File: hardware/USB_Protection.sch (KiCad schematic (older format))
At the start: 10 parts, among them Q1 DMN6140L, U12 TCPP01-M12

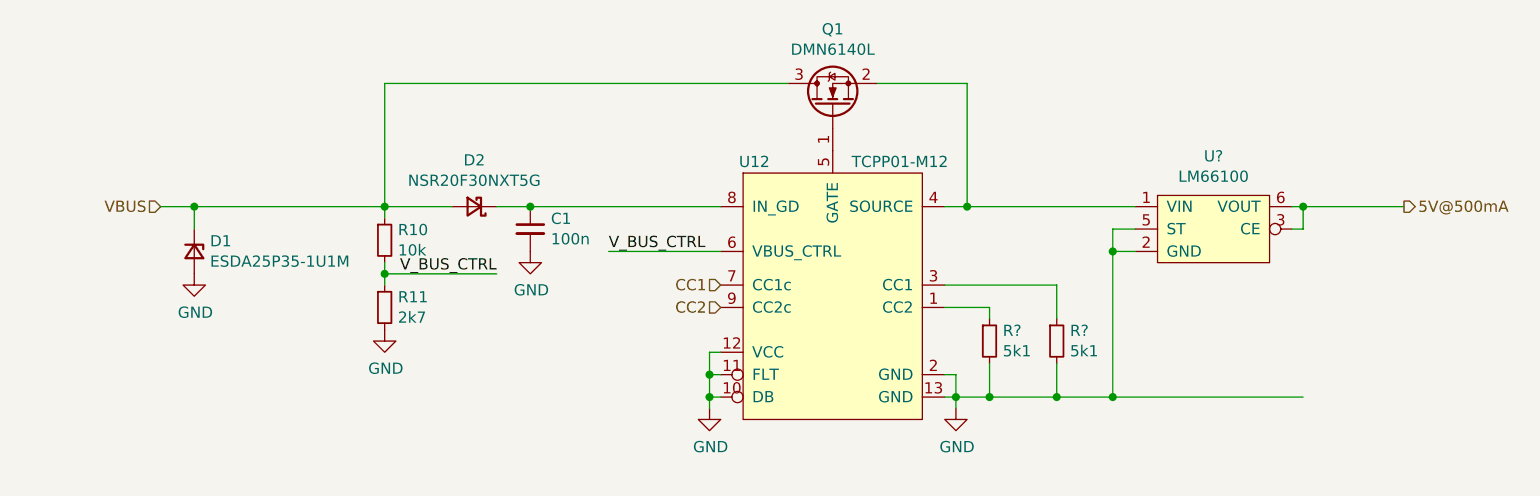
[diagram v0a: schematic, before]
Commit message: hardware development
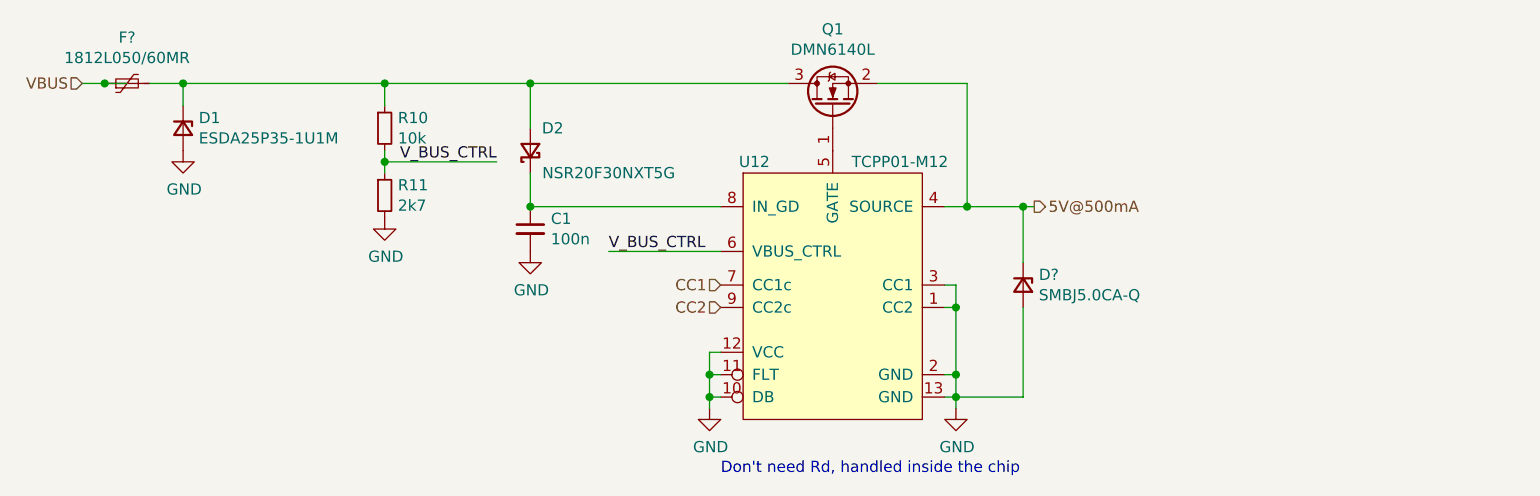
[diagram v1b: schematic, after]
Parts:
- removed R? (x2): 5k1, Resistor_SMD:R_0603_1608Metric_Pad1.05x0.95mm_HandSolder, symbol Device:R_Small
- removed U?: LM66100, lm66100:LM66100DCKT, symbol watch:LM66100-Variant2
- added D?: SMBJ5.0CA-Q, Diode_SMD:D_0603_1608Metric_Pad1.05x0.95mm_HandSolder, symbol Device:D_Zener_Small
- added F?: 1812L050/60MR, symbol Device:Polyfuse_Small
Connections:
- wire segments 45 -> 37
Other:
- note added: "Don't need Rd, handled inside the chip"
- moved on the sheet: D1, D2, R10, R11
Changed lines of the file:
@@
 $Descr A4 11693 8268
 encoding utf-8
-Sheet 2 3
+Sheet 3 4
 Title ""
 Date ""
@@
 AR Path="/6072C21E" Ref="U?"  Part="1"
 AR Path="/6071FFAF/6072C21E" Ref="U12"  Part="1"
+AR Path="/60604F0C/6060934C/6072C21E" Ref="U?"  Part="1"
 F 0 "U12" H 4650 3750 50  0000 C CNN
 F 1 "TCPP01-M12" H 5300 3750 50  0000 C CNN
@@
 L Device:D_Zener_Small D?
 U 1 1 60731C37
-P 2150 2950
+P 2100 2400
 AR Path="/60731C37" Ref="D?"  Part="1"
 AR Path="/6071FFAF/60731C37" Ref="D1"  Part="1"
-F 0 "D1" V 2104 3020 50  0000 L CNN
-F 1 "ESDA25P35-1U1M" V 2195 3020 50  0000 L CNN
-F 2 "Diode_SMD:D_0603_1608Metric_Pad1.05x0.95mm_HandSolder" V 2150 2950 50  0001 C CNN
-F 3 "~" V 2150 2950 50  0001 C CNN
-	1    2150 2950
+AR Path="/60604F0C/6060934C/60731C37" Ref="D?"  Part="1"
+F 0 "D1" V 2054 2470 50  0000 L CNN
+F 1 "ESDA25P35-1U1M" V 2145 2470 50  0000 L CNN
+F 2 "Diode_SMD:D_0603_1608Metric_Pad1.05x0.95mm_HandSolder" V 2100 2400 50  0001 C CNN
+F 3 "~" V 2100 2400 50  0001 C CNN
+	1    2100 2400
 	0    1    1    0
 $EndComp
-Text HLabel 2000 2750 0    50   Input ~ 0
+Text HLabel 1650 2200 0    50   Input ~ 0
 VBUS
 Text HLabel 4500 3100 0    50   Input ~ 0
@@
 U 1 1 605BE08D
 P 5550 3650
+AR Path="/6071FFAF/605BE08D" Ref="#PWR0130"  Part="1"
+AR Path="/60604F0C/6060934C/605BE08D" Ref="#PWR?"  Part="1"
 F 0 "#PWR0130" H 5550 3400 50  0001 C CNN
 F 1 "GND" H 5555 3477 50  0000 C CNN
@@
 U 1 1 605BEA49
 P 4450 3650
+AR Path="/6071FFAF/605BEA49" Ref="#PWR0131"  Part="1"
+AR Path="/60604F0C/6060934C/605BEA49" Ref="#PWR?"  Part="1"
 F 0 "#PWR0131" H 4450 3400 50  0001 C CNN
 F 1 "GND" H 4455 3477 50  0000 C CNN
@@
 	4450 3600 4450 3500
 Wire Wire Line
-	2150 2850 2150 2750
-Wire Wire Line
-	2150 2750 2000 2750
+	2100 2300 2100 2200
 $Comp
 L Device:R_Small R10
 U 1 1 605BF926
-P 3000 2900
-F 0 "R10" H 3059 2946 50  0000 L CNN
-F 1 "10k" H 3059 2855 50  0000 L CNN
-F 2 "Resistor_SMD:R_0603_1608Metric_Pad1.05x0.95mm_HandSolder" H 3000 2900 50  0001 C CNN
-F 3 "~" H 3000 2900 50  0001 C CNN
-	1    3000 2900
+P 3000 2400
+AR Path="/6071FFAF/605BF926" Ref="R10"  Part="1"
+AR Path="/60604F0C/6060934C/605BF926" Ref="R?"  Part="1"
+F 0 "R10" H 3059 2446 50  0000 L CNN
+F 1 "10k" H 3059 2355 50  0000 L CNN
+F 2 "Resistor_SMD:R_0603_1608Metric_Pad1.05x0.95mm_HandSolder" H 3000 2400 50  0001 C CNN
+F 3 "~" H 3000 2400 50  0001 C CNN
+	1    3000 2400
 	1    0    0    -1
 $EndComp
@@
 L Device:R_Small R11
 U 1 1 605C0410
-P 3000 3200
-F 0 "R11" H 3059 3246 50  0000 L CNN
-F 1 "2k7" H 3059 3155 50  0000 L CNN
-F 2 "Resistor_SMD:R_0603_1608Metric_Pad1.05x0.95mm_HandSolder" H 3000 3200 50  0001 C CNN
-F 3 "~" H 3000 3200 50  0001 C CNN
-	1    3000 3200
-	1    0    0    -1
-$EndComp
-Wire Wire Line
-	2150 2750 3000 2750
-Wire Wire Line
-	3000 2750 3000 2800
-Connection ~ 2150 2750
+P 3000 2700
+AR Path="/6071FFAF/605C0410" Ref="R11"  Part="1"
+AR Path="/60604F0C/6060934C/605C0410" Ref="R?"  Part="1"
+F 0 "R11" H 3059 2746 50  0000 L CNN
+F 1 "2k7" H 3059 2655 50  0000 L CNN
+F 2 "Resistor_SMD:R_0603_1608Metric_Pad1.05x0.95mm_HandSolder" H 3000 2700 50  0001 C CNN
+F 3 "~" H 3000 2700 50  0001 C CNN
+	1    3000 2700
+	1    0    0    -1
+$EndComp
 $Comp
 L Device:D_Schottky_Small D2
 U 1 1 605C65BD
-P 3400 2750
-F 0 "D2" H 3400 2543 50  0000 C CNN
-F 1 "NSR20F30NXT5G" H 3400 2634 50  0000 C CNN
-F 2 "Diode_SMD:D_0603_1608Metric_Pad1.05x0.95mm_HandSolder" V 3400 2750 50  0001 C CNN
-F 3 "~" V 3400 2750 50  0001 C CNN
-	1    3400 2750
-	-1   0    0    1
+P 3650 2500
+AR Path="/6071FFAF/605C65BD" Ref="D2"  Part="1"
+AR Path="/60604F0C/6060934C/605C65BD" Ref="D?"  Part="1"
+F 0 "D2" V 3750 2400 50  0000 C CNN
+F 1 "NSR20F30NXT5G" V 3550 2150 50  0000 C CNN
+F 2 "Diode_SMD:D_0603_1608Metric_Pad1.05x0.95mm_HandSolder" V 3650 2500 50  0001 C CNN
+F 3 "~" V 3650 2500 50  0001 C CNN
+	1    3650 2500
+	0    -1   -1   0
 $EndComp
 $Comp
@@
 U 1 1 605C70FD
 P 3650 2850
+AR Path="/6071FFAF/605C70FD" Ref="C1"  Part="1"
+AR Path="/60604F0C/6060934C/605C70FD" Ref="C?"  Part="1"
 F 0 "C1" H 3742 2896 50  0000 L CNN
 F 1 "100n" H 3742 2805 50  0000 L CNN
@@
 L power:GND #PWR0132
 U 1 1 605BDB68
-P 2150 3050
-F 0 "#PWR0132" H 2150 2800 50  0001 C CNN
-F 1 "GND" H 2155 2877 50  0000 C CNN
-F 2 "" H 2150 3050 50  0001 C CNN
-F 3 "" H 2150 3050 50  0001 C CNN
-	1    2150 3050
+P 2100 2500
+AR Path="/6071FFAF/605BDB68" Ref="#PWR0132"  Part="1"
+AR Path="/60604F0C/6060934C/605BDB68" Ref="#PWR?"  Part="1"
+F 0 "#PWR0132" H 2100 2250 50  0001 C CNN
+F 1 "GND" H 2105 2327 50  0000 C CNN
+F 2 "" H 2100 2500 50  0001 C CNN
+F 3 "" H 2100 2500 50  0001 C CNN
+	1    2100 2500
 	1    0    0    -1
 $EndComp
@@
 L power:GND #PWR0133
 U 1 1 605C1A8E
-P 3000 3300
-F 0 "#PWR0133" H 3000 3050 50  0001 C CNN
-F 1 "GND" H 3005 3127 50  0000 C CNN
-F 2 "" H 3000 3300 50  0001 C CNN
-F 3 "" H 3000 3300 50  0001 C CNN
-	1    3000 3300
-	1    0    0    -1
-$EndComp
-Wire Wire Line
-	3000 3000 3000 3050
-Wire Wire Line
-	3300 2750 3000 2750
-Connection ~ 3000 2750
+P 3000 2800
+AR Path="/6071FFAF/605C1A8E" Ref="#PWR0133"  Part="1"
+AR Path="/60604F0C/6060934C/605C1A8E" Ref="#PWR?"  Part="1"
+F 0 "#PWR0133" H 3000 2550 50  0001 C CNN
+F 1 "GND" H 3005 2627 50  0000 C CNN
+F 2 "" H 3000 2800 50  0001 C CNN
+F 3 "" H 3000 2800 50  0001 C CNN
+	1    3000 2800
+	1    0    0    -1
+$EndComp
+Wire Wire Line
+	3000 2500 3000 2550
 $Comp
 L power:GND #PWR0136
 U 1 1 605CCB83
 P 3650 2950
+AR Path="/6071FFAF/605CCB83" Ref="#PWR0136"  Part="1"
+AR Path="/60604F0C/6060934C/605CCB83" Ref="#PWR?"  Part="1"
 F 0 "#PWR0136" H 3650 2700 50  0001 C CNN
 F 1 "GND" H 3655 2777 50  0000 C CNN
@@
 	1    0    0    -1
 $EndComp
-Wire Wire Line
-	3500 2750 3650 2750
-Connection ~ 3650 2750
-Text Label 3500 3050 2    50   ~ 0
+Text Label 3500 2550 2    50   ~ 0
 V_BUS_CTRL
 Wire Wire Line
-	3500 3050 3000 3050
-Connection ~ 3000 3050
-Wire Wire Line
-	3000 3050 3000 3100
+	3500 2550 3000 2550
+Connection ~ 3000 2550
+Wire Wire Line
+	3000 2550 3000 2600
 Text Label 4000 2950 0    50   ~ 0
 V_BUS_CTRL
@@
 U 1 1 605D3F9F
 P 5000 2300
+AR Path="/6071FFAF/605D3F9F" Ref="Q1"  Part="1"
+AR Path="/60604F0C/6060934C/605D3F9F" Ref="Q?"  Part="1"
 F 0 "Q1" V 5342 2300 50  0000 C CNN
 F 1 "DMN6140L" V 5251 2300 50  0000 C CNN
@@
 Wire Wire Line
 	5600 2750 5500 2750
-Text HLabel 7550 2750 2    50   Output ~ 0
+Text HLabel 5900 2750 2    50   Output ~ 0
 5V@500mA
 Connection ~ 5600 2750
@@
 	3650 2750 4500 2750
 Wire Wire Line
-	3000 2200 3000 2750
-Wire Wire Line
-	3000 2200 4800 2200
-$Comp
-L Device:R_Small R?
-U 1 1 605C8234
-P 5700 3350
-F 0 "R?" H 5759 3396 50  0000 L CNN
-F 1 "5k1" H 5759 3305 50  0000 L CNN
-F 2 "Resistor_SMD:R_0603_1608Metric_Pad1.05x0.95mm_HandSolder" H 5700 3350 50  0001 C CNN
-F 3 "~" H 5700 3350 50  0001 C CNN
-	1    5700 3350
-	1    0    0    -1
-$EndComp
-$Comp
-L Device:R_Small R?
-U 1 1 605C8525
-P 6000 3350
-F 0 "R?" H 6059 3396 50  0000 L CNN
-F 1 "5k1" H 6059 3305 50  0000 L CNN
-F 2 "Resistor_SMD:R_0603_1608Metric_Pad1.05x0.95mm_HandSolder" H 6000 3350 50  0001 C CNN
-F 3 "~" H 6000 3350 50  0001 C CNN
-	1    6000 3350
-	1    0    0    -1
-$EndComp
-Wire Wire Line
-	5700 3200 5700 3250
-Wire Wire Line
-	5500 3200 5700 3200
-Wire Wire Line
-	6000 3100 6000 3250
-Wire Wire Line
-	5500 3100 6000 3100
-Wire Wire Line
-	5700 3450 5700 3600
-Wire Wire Line
-	5700 3600 5550 3600
-Wire Wire Line
-	6000 3450 6000 3600
-Wire Wire Line
-	6000 3600 5700 3600
-Connection ~ 5700 3600
-Wire Wire Line
-	5600 2750 6350 2750
-Wire Wire Line
-	6350 2950 6250 2950
-Wire Wire Line
-	6250 2950 6250 3600
-Wire Wire Line
-	6250 3600 6000 3600
-Connection ~ 6000 3600
-Wire Wire Line
-	7100 3600 6250 3600
-Connection ~ 6250 3600
-$Comp
-L watch:LM66100-Variant2 U?
-U 1 1 605D85BE
-P 6700 2850
-F 0 "U?" H 6700 3175 50  0000 C CNN
-F 1 "LM66100" H 6700 3084 50  0000 C CNN
-F 2 "lm66100:LM66100DCKT" H 7050 3100 50  0001 C CNN
-F 3 "" H 7050 3100 50  0001 C CNN
-	1    6700 2850
-	1    0    0    -1
-$EndComp
-Wire Wire Line
-	7050 2750 7100 2750
-Wire Wire Line
-	6350 2850 6250 2850
-Wire Wire Line
-	6250 2850 6250 2950
-Connection ~ 6250 2950
-Wire Wire Line
-	7050 2850 7100 2850
-Wire Wire Line
-	7100 2850 7100 2750
-Connection ~ 7100 2750
-Wire Wire Line
-	7100 2750 7550 2750
+	3000 2200 3650 2200
+Wire Wire Line
+	5600 2750 5850 2750
+Wire Wire Line
+	5550 3600 5850 3600
+Wire Wire Line
+	5550 3500 5550 3200
+Wire Wire Line
+	5550 3100 5500 3100
+Connection ~ 5550 3500
+Wire Wire Line
+	5500 3200 5550 3200
+Connection ~ 5550 3200
+Wire Wire Line
+	5550 3200 5550 3100
+$Comp
+L Device:D_Zener_Small D?
+U 1 1 605F2ABA
+P 5850 3100
+AR Path="/605F2ABA" Ref="D?"  Part="1"
+AR Path="/6071FFAF/605F2ABA" Ref="D?"  Part="1"
+AR Path="/60604F0C/6060934C/605F2ABA" Ref="D?"  Part="1"
+F 0 "D?" V 5804 3170 50  0000 L CNN
+F 1 "SMBJ5.0CA-Q" V 5895 3170 50  0000 L CNN
+F 2 "Diode_SMD:D_0603_1608Metric_Pad1.05x0.95mm_HandSolder" V 5850 3100 50  0001 C CNN
+F 3 "~" V 5850 3100 50  0001 C CNN
+	1    5850 3100
+	0    1    1    0
+$EndComp
+Wire Wire Line
+	5850 2750 5850 3000
+Wire Wire Line
+	5850 3200 5850 3600
+Text Notes 4500 3950 0    50   ~ 0
+Don't need Rd, handled inside the chip
+$Comp
+L Device:Polyfuse_Small F?
+U 1 1 6064BF52
+P 1850 2200
+F 0 "F?" V 2055 2200 50  0000 C CNN
+F 1 "1812L050/60MR" V 1964 2200 50  0000 C CNN
+F 2 "" H 1900 2000 50  0001 L CNN
+F 3 "~" H 1850 2200 50  0001 C CNN
+	1    1850 2200
+	0    -1   -1   0
+$EndComp
+Wire Wire Line
+	1950 2200 2100 2200
+Wire Wire Line
+	1850 2200 1750 2200
+Wire Wire Line
+	3650 2400 3650 2200
+Connection ~ 3650 2200
+Wire Wire Line
+	3650 2200 4800 2200
+Wire Wire Line
+	3650 2600 3650 2750
+Connection ~ 3650 2750
+Connection ~ 1750 2200
+Wire Wire Line
+	1750 2200 1650 2200
+Wire Wire Line
+	3000 2200 3000 2300
+Wire Wire Line
+	3000 2200 2100 2200
+Connection ~ 3000 2200
+Connection ~ 2100 2200
+Wire Wire Line
+	5900 2750 5850 2750
+Connection ~ 5850 2750
 $EndSCHEMATC
